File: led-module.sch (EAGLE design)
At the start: 36 parts, among them U1 LT3956EUHEPBFUHE_36_ADI-M, U2 RUR020N02TL

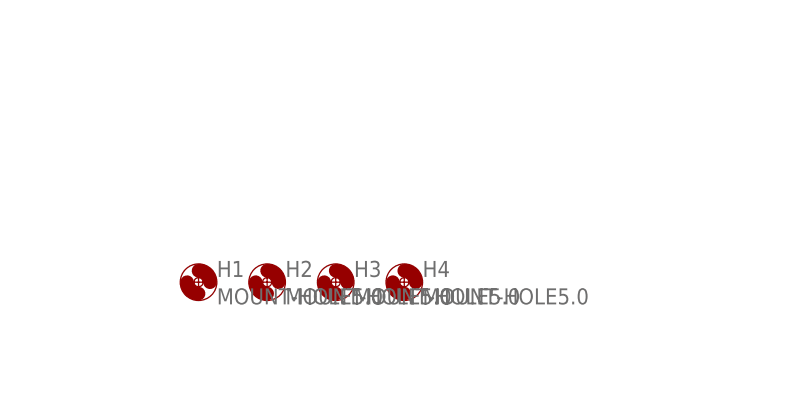
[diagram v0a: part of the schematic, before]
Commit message: Added libraries
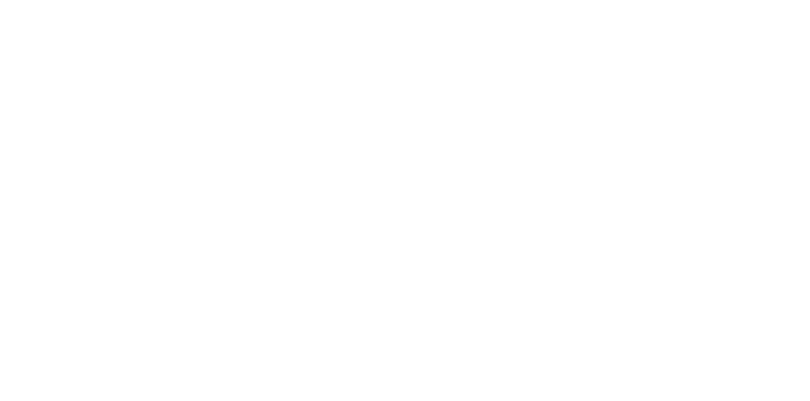
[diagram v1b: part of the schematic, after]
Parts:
- removed H1, H2, H3, H4: MOUNT-HOLE5.0, holes:MOUNT-HOLE5.0
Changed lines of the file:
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@@
 <part name="C6" library="rcl" library_urn="urn:adsk.eagle:library:334" deviceset="C-EU" device="C0805" package3d_urn="urn:adsk.eagle:package:23617/2" value="10uF"/>
 <part name="U$1" library="5-2154874-3" deviceset="5-2154874-3" device=""/>
-<part name="H1" library="holes" library_urn="urn:adsk.eagle:library:237" deviceset="MOUNT-HOLE" device="5.0" package3d_urn="urn:adsk.eagle:package:14276/1"/>
-<part name="H2" library="holes" library_urn="urn:adsk.eagle:library:237" deviceset="MOUNT-HOLE" device="5.0" package3d_urn="urn:adsk.eagle:package:14276/1"/>
-<part name="H3" library="holes" library_urn="urn:adsk.eagle:library:237" deviceset="MOUNT-HOLE" device="5.0" package3d_urn="urn:adsk.eagle:package:14276/1"/>
-<part name="H4" library="holes" library_urn="urn:adsk.eagle:library:237" deviceset="MOUNT-HOLE" device="5.0" package3d_urn="urn:adsk.eagle:package:14276/1"/>
 </parts>
 <sheets>
@@
 <attribute name="NAME" x="260.096" y="-12.192" size="1.778" layer="95" rot="R90"/>
 </instance>
-<instance part="H1" gate="G$1" x="149.86" y="-78.74" smashed="yes">
-<attribute name="NAME" x="151.892" y="-78.1558" size="1.778" layer="95"/>
-<attribute name="VALUE" x="151.892" y="-81.2038" size="1.778" layer="96"/>
-</instance>
-<instance part="H2" gate="G$1" x="157.48" y="-78.74" smashed="yes">
-<attribute name="NAME" x="159.512" y="-78.1558" size="1.778" layer="95"/>
-<attribute name="VALUE" x="159.512" y="-81.2038" size="1.778" layer="96"/>
-</instance>
-<instance part="H3" gate="G$1" x="165.1" y="-78.74" smashed="yes">
-<attribute name="NAME" x="167.132" y="-78.1558" size="1.778" layer="95"/>
-<attribute name="VALUE" x="167.132" y="-81.2038" size="1.778" layer="96"/>
-</instance>
-<instance part="H4" gate="G$1" x="172.72" y="-78.74" smashed="yes">
-<attribute name="NAME" x="174.752" y="-78.1558" size="1.778" layer="95"/>
-<attribute name="VALUE" x="174.752" y="-81.2038" size="1.778" layer="96"/>
-</instance>
 </instances>
